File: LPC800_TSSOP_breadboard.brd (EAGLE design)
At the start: 31.4 x 15.8 mm, 17 parts, among them Q1 12MHz

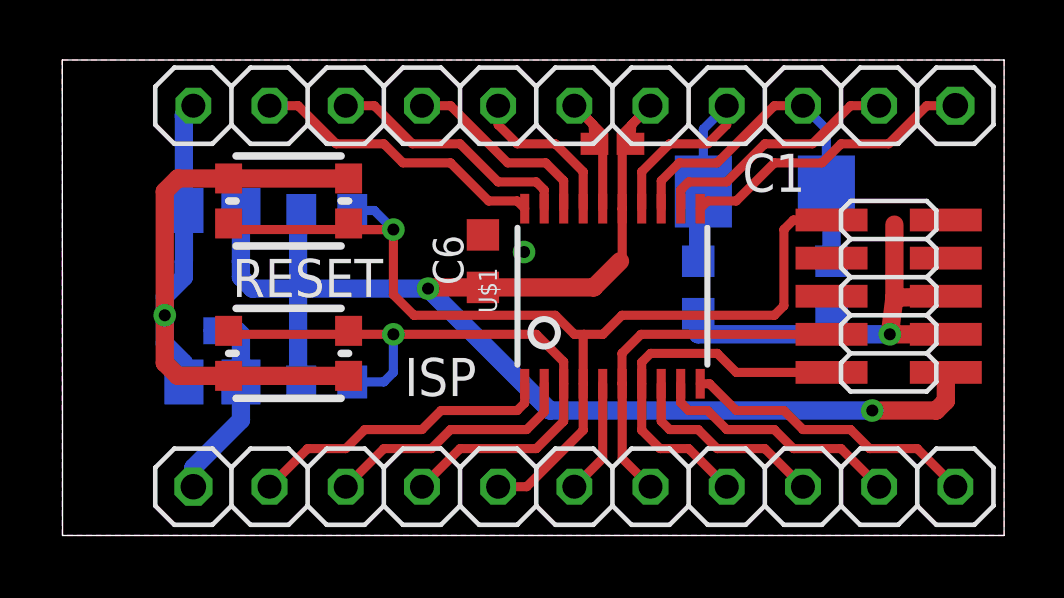
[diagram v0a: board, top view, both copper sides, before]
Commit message: * updated board and schem with todo's
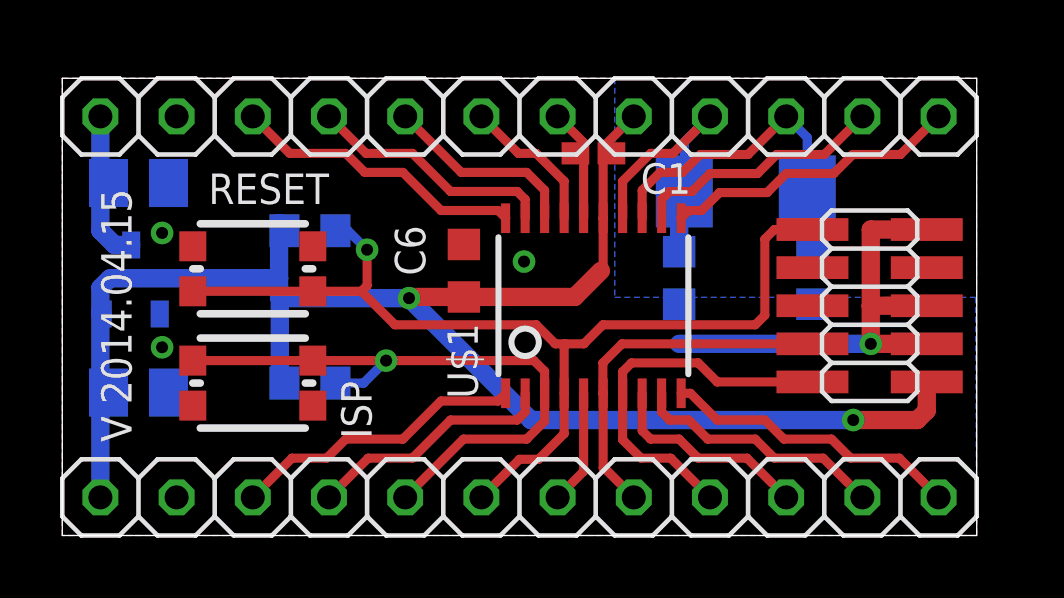
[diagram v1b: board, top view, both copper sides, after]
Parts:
- removed JP1, JP2: (no value), bart_connectors:1X11_SMALL
- removed LOGO1: OSHW_LOGO_FILLX0150-NT, ohw-logo:OSHW_FILLX150_NOTEXT
- added JP4, JP5: (no value), SquantorConnectors:1X12_SMALL
- added LOGO2: OSHW_LOGO_FILLX0150-NT, ohw-logo:OSHW_FILLX150_NOTEXT
- C4, C5: device bart_rcl:C0805 -> bart_rcl:C0805K
- moved C5 7.07 mm to (2.54, 11.7), turned to 180 degrees
- moved C4 6.55 mm to (2.54, 4.76), turned to 180 degrees
- moved U$2 2.76 mm to (2.30, 8.53), turned to 0 degrees
- moved U$3 2.56 mm to (6.35, 8.89)
- moved U$4 1.55 mm to (6.35, 5.08)
- moved R2 0.87 mm to (8.26, 10.2)
- moved C2 0.71 mm to (20.6, 8.59)
- moved C3 0.71 mm to (25.0, 8.59)
- moved C6 0.71 mm to (13.4, 8.83)
- moved C1 0.71 mm to (17.7, 12.7)
- moved JP3 0.71 mm to (26.9, 7.66)
- moved U$1 0.71 mm to (17.7, 7.66)
- moved Q1 0.64 mm to (22.8, 11.5)
- moved R1 0.56 mm to (8.26, 5.08)
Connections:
- net PIO0_0: now also JP4.9; no longer JP1.9
- net PIO0_1: now also JP4.2; no longer JP1.2
- net PIO0_10: now also JP5.11; no longer JP2.10
- net PIO0_11: now also JP5.10; no longer JP2.9
- net PIO0_12: now also JP5.5; no longer JP2.4
- net PIO0_13: now also JP5.4; no longer JP2.3
- net PIO0_14: now also JP4.10; no longer JP1.10
- net PIO0_15: now also JP4.1; no longer JP1.1
- net PIO0_16: now also JP5.12; no longer JP2.11
- net PIO0_17: now also JP5.3; no longer JP2.2
- net PIO0_2: now also JP5.9; no longer JP2.8
- net PIO0_3: now also JP5.8; no longer JP2.7
- net PIO0_4: now also JP5.7; no longer JP2.6
- net PIO0_5: now also JP5.6; no longer JP2.5
- net PIO0_6: now also JP4.8; no longer JP1.8
- net PIO0_7: now also JP4.7; no longer JP1.7
- net PIO0_8: now also JP4.4; no longer JP1.4
- net PIO0_9: now also JP4.3; no longer JP1.3
- net VCCIO: now also JP4.12; no longer JP2.1
- net VDD: now also JP4.5, JP5.1; no longer JP1.5
- net VSS: now also JP4.11, JP4.6, JP5.2; no longer JP1.11, JP1.6
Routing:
- net VSS: track 48.6 -> 19.8 mm, vias 3 -> 4
- net VDD: track 48.4 -> 56.0 mm
- net PIO0_5: track 36.2 -> 33.9 mm
- net VCCIO: track 6.74 -> 5.31 mm
- net PIO0_12: track 22.3 -> 21.2 mm
- net PIO0_8: track 10.9 -> 9.92 mm
- net PIO0_9: track 12.2 -> 11.6 mm
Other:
- board size 31.4 x 15.8 mm -> 30.5 x 15.2 mm
